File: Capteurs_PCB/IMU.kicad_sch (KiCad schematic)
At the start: 1 part, among them U3 LSM6DSL

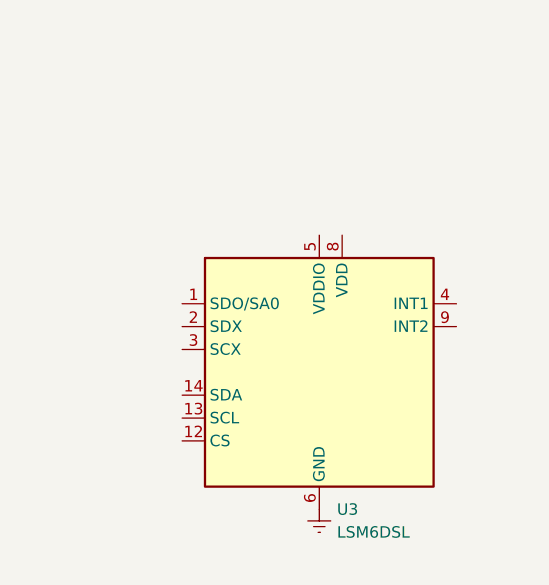
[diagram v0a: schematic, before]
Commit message: pcb update
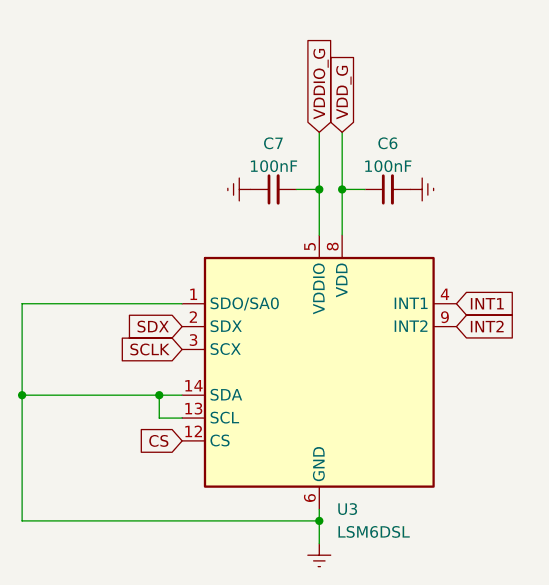
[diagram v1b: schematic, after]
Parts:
- added C6, C7: 100nF, symbol Device:C_Small
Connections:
- net Earth: now also U3.1 (SDO/SA0), U3.13 (SCL), U3.14 (SDA), C6.2, C7.1
- net CS: now reaches U3.12 (CS)
- net SDX: now reaches U3.2 (SDX)
- net SCLK: now reaches U3.3 (SCX)
- net INT1: now reaches U3.4 (INT1)
- net VDDIO_G: now reaches U3.5 (VDDIO)
- net VDDIO_G: now also C7.2
- net VDD_G: now reaches U3.8 (VDD)
- net VDD_G: now also C6.1
- net INT2: now reaches U3.9 (INT2)
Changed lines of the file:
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@@
 (kicad_sch (version 20230121) (generator eeschema)
   (paper "A4")
-  (symbol (lib_id "power:Earth") (at 137.16 95.25 0) (unit 1)
-    (in_bom yes) (on_board yes) (dnp no) (fields_autoplaced)
-    (property "Reference" "#PWR03" (at 137.16 101.6 0)
-      (effects (font (size 1.27 1.27)) hide)
-    )
-    (property "Value" "Earth" (at 137.16 99.06 0)
-      (effects (font (size 1.27 1.27)) hide)
-    )
-    (property "Footprint" "" (at 137.16 95.25 0)
-      (effects (font (size 1.27 1.27)) hide)
-    )
-    (property "Datasheet" "~" (at 137.16 95.25 0)
+  (junction (at 137.16 59.69) (diameter 0) (color 0 0 0 0)
+  )
+  (junction (at 104.14 82.55) (diameter 0) (color 0 0 0 0)
+  )
+  (junction (at 137.16 96.52) (diameter 0) (color 0 0 0 0)
+  )
+  (junction (at 119.38 82.55) (diameter 0) (color 0 0 0 0)
+  )
+  (junction (at 139.7 59.69) (diameter 0) (color 0 0 0 0)
+  )
+  (wire (pts (xy 104.14 96.52) (xy 137.16 96.52))
+    (stroke (width 0) (type default))
+  )
+  (wire (pts (xy 139.7 53.34) (xy 139.7 59.69))
+    (stroke (width 0) (type default))
+  )
+  (wire (pts (xy 121.92 85.09) (xy 119.38 85.09))
+    (stroke (width 0) (type default))
+  )
+  (wire (pts (xy 119.38 85.09) (xy 119.38 82.55))
+    (stroke (width 0) (type default))
+  )
+  (wire (pts (xy 139.7 59.69) (xy 142.24 59.69))
+    (stroke (width 0) (type default))
+  )
+  (wire (pts (xy 137.16 95.25) (xy 137.16 96.52))
+    (stroke (width 0) (type default))
+  )
+  (wire (pts (xy 104.14 82.55) (xy 104.14 96.52))
+    (stroke (width 0) (type default))
+  )
+  (wire (pts (xy 104.14 82.55) (xy 119.38 82.55))
+    (stroke (width 0) (type default))
+  )
+  (wire (pts (xy 121.92 72.39) (xy 104.14 72.39))
+    (stroke (width 0) (type default))
+  )
+  (wire (pts (xy 137.16 59.69) (xy 134.62 59.69))
+    (stroke (width 0) (type default))
+  )
+  (wire (pts (xy 119.38 82.55) (xy 121.92 82.55))
+    (stroke (width 0) (type default))
+  )
+  (wire (pts (xy 104.14 72.39) (xy 104.14 82.55))
+    (stroke (width 0) (type default))
+  )
+  (wire (pts (xy 137.16 96.52) (xy 137.16 99.06))
+    (stroke (width 0) (type default))
+  )
+  (wire (pts (xy 139.7 59.69) (xy 139.7 64.77))
+    (stroke (width 0) (type default))
+  )
+  (wire (pts (xy 137.16 59.69) (xy 137.16 64.77))
+    (stroke (width 0) (type default))
+  )
+  (wire (pts (xy 137.16 53.34) (xy 137.16 59.69))
+    (stroke (width 0) (type default))
+  )
+  (global_label "SDX" (shape input) (at 121.92 74.93 180) (fields_autoplaced)
+    (effects (font (size 1.27 1.27)) (justify right))
+    (property "Intersheetrefs" "${INTERSHEET_REFS}" (at 115.3252 74.93 0)
+      (effects (font (size 1.27 1.27)) (justify right) hide)
+    )
+  )
+  (global_label "INT1" (shape input) (at 152.4 72.39 0) (fields_autoplaced)
+    (effects (font (size 1.27 1.27)) (justify left))
+    (property "Intersheetrefs" "${INTERSHEET_REFS}" (at 159.4182 72.39 0)
+      (effects (font (size 1.27 1.27)) (justify left) hide)
+    )
+  )
+  (global_label "SCLK" (shape input) (at 121.92 77.47 180) (fields_autoplaced)
+    (effects (font (size 1.27 1.27)) (justify right))
+    (property "Intersheetrefs" "${INTERSHEET_REFS}" (at 114.2366 77.47 0)
+      (effects (font (size 1.27 1.27)) (justify right) hide)
+    )
+  )
+  (global_label "VDD_G" (shape input) (at 139.7 53.34 90) (fields_autoplaced)
+    (effects (font (size 1.27 1.27)) (justify left))
+    (property "Intersheetrefs" "${INTERSHEET_REFS}" (at 139.7 44.568 90)
+      (effects (font (size 1.27 1.27)) (justify left) hide)
+    )
+  )
+  (global_label "INT2" (shape input) (at 152.4 74.93 0) (fields_autoplaced)
+    (effects (font (size 1.27 1.27)) (justify left))
+    (property "Intersheetrefs" "${INTERSHEET_REFS}" (at 159.4182 74.93 0)
+      (effects (font (size 1.27 1.27)) (justify left) hide)
+    )
+  )
+  (global_label "VDDIO_G" (shape input) (at 137.16 53.34 90) (fields_autoplaced)
+    (effects (font (size 1.27 1.27)) (justify left))
+    (property "Intersheetrefs" "${INTERSHEET_REFS}" (at 137.16 42.6327 90)
+      (effects (font (size 1.27 1.27)) (justify left) hide)
+    )
+  )
+  (global_label "CS" (shape input) (at 121.92 87.63 180) (fields_autoplaced)
+    (effects (font (size 1.27 1.27)) (justify right))
+    (property "Intersheetrefs" "${INTERSHEET_REFS}" (at 116.5347 87.63 0)
+      (effects (font (size 1.27 1.27)) (justify right) hide)
+    )
+  )
+  (symbol (lib_id "power:Earth") (at 137.16 99.06 0) (unit 1)
+    (in_bom yes) (on_board yes) (dnp no) (fields_autoplaced)
+    (property "Reference" "#PWR03" (at 137.16 105.41 0)
+      (effects (font (size 1.27 1.27)) hide)
+    )
+    (property "Value" "Earth" (at 137.16 102.87 0)
+      (effects (font (size 1.27 1.27)) hide)
+    )
+    (property "Footprint" "" (at 137.16 99.06 0)
+      (effects (font (size 1.27 1.27)) hide)
+    )
+    (property "Datasheet" "~" (at 137.16 99.06 0)
       (effects (font (size 1.27 1.27)) hide)
     )
@@
         )
       )
+    )
+  )
+  (symbol (lib_id "Device:C_Small") (at 144.78 59.69 90) (unit 1)
+    (in_bom yes) (on_board yes) (dnp no) (fields_autoplaced)
+    (property "Reference" "C6" (at 144.7863 54.61 90)
+      (effects (font (size 1.27 1.27)))
+    )
+    (property "Value" "100nF" (at 144.7863 57.15 90)
+      (effects (font (size 1.27 1.27)))
+    )
+    (property "Footprint" "" (at 144.78 59.69 0)
+      (effects (font (size 1.27 1.27)) hide)
+    )
+    (property "Datasheet" "~" (at 144.78 59.69 0)
+      (effects (font (size 1.27 1.27)) hide)
+    )
+    (pin "1")
+    (pin "2")
+    (instances
+      (project "Capteurs_PCB"
+        (path "/1101af8f-9425-4102-9245-339dc54562bf/5a49e44b-df85-4cd7-b98e-18311503a9a2"
+          (reference "C6") (unit 1)
+        )
+      )
+    )
+  )
+  (symbol (lib_id "Device:C_Small") (at 132.08 59.69 90) (unit 1)
+    (in_bom yes) (on_board yes) (dnp no) (fields_autoplaced)
+    (property "Reference" "C7" (at 132.0863 54.61 90)
+      (effects (font (size 1.27 1.27)))
+    )
+    (property "Value" "100nF" (at 132.0863 57.15 90)
+      (effects (font (size 1.27 1.27)))
+    )
+    (property "Footprint" "" (at 132.08 59.69 0)
+      (effects (font (size 1.27 1.27)) hide)
+    )
+    (property "Datasheet" "~" (at 132.08 59.69 0)
+      (effects (font (size 1.27 1.27)) hide)
+    )
+    (pin "1")
+    (pin "2")
+    (instances
+      (project "Capteurs_PCB"
+        (path "/1101af8f-9425-4102-9245-339dc54562bf/5a49e44b-df85-4cd7-b98e-18311503a9a2"
+          (reference "C7") (unit 1)
+        )
+      )
+    )
+  )
+  (symbol (lib_id "power:Earth") (at 129.54 59.69 270) (unit 1)
+    (in_bom yes) (on_board yes) (dnp no) (fields_autoplaced)
+    (property "Reference" "#PWR07" (at 123.19 59.69 0)
+      (effects (font (size 1.27 1.27)) hide)
+    )
+    (property "Value" "Earth" (at 125.73 59.69 0)
+      (effects (font (size 1.27 1.27)) hide)
+    )
+    (property "Footprint" "" (at 129.54 59.69 0)
+      (effects (font (size 1.27 1.27)) hide)
+    )
+    (property "Datasheet" "~" (at 129.54 59.69 0)
+      (effects (font (size 1.27 1.27)) hide)
+    )
+    (pin "1")
+    (instances
+      (project "Capteurs_PCB"
+        (path "/1101af8f-9425-4102-9245-339dc54562bf/5a49e44b-df85-4cd7-b98e-18311503a9a2"
+          (reference "#PWR07") (unit 1)
+        )
+      )
+    )
+  )
+  (symbol (lib_id "power:Earth") (at 147.32 59.69 90) (unit 1)
+    (in_bom yes) (on_board yes) (dnp no) (fields_autoplaced)
+    (property "Reference" "#PWR05" (at 153.67 59.69 0)
+      (effects (font (size 1.27 1.27)) hide)
+    )
+    (property "Value" "Earth" (at 151.13 59.69 0)
+      (effects (font (size 1.27 1.27)) hide)
+    )
+    (property "Footprint" "" (at 147.32 59.69 0)
+      (effects (font (size 1.27 1.27)) hide)
+    )
+    (property "Datasheet" "~" (at 147.32 59.69 0)
+      (effects (font (size 1.27 1.27)) hide)
+    )
+    (pin "1")
+    (instances
+      (project "Capteurs_PCB"
+        (path "/1101af8f-9425-4102-9245-339dc54562bf/5a49e44b-df85-4cd7-b98e-18311503a9a2"
+          (reference "#PWR05") (unit 1)
+        )
+      )

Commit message: updates pcb
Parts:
- C6, C7: footprint (none) -> Capacitor_SMD:C_1206_3216Metric
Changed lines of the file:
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@@
       (effects (font (size 1.27 1.27)))
     )
-    (property "Footprint" "" (at 144.78 59.69 0)
+    (property "Footprint" "Capacitor_SMD:C_1206_3216Metric" (at 144.78 59.69 0)
       (effects (font (size 1.27 1.27)) hide)
     )
@@
       (effects (font (size 1.27 1.27)))
     )
-    (property "Footprint" "" (at 132.08 59.69 0)
+    (property "Footprint" "Capacitor_SMD:C_1206_3216Metric" (at 132.08 59.69 0)
       (effects (font (size 1.27 1.27)) hide)
     )
